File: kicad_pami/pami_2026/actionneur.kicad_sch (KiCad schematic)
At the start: 18 parts, among them J1 Conn_01x04_Socket, J10 Conn_01x07_Socket, J11 Conn_01x06, J12 Conn_01x06, J14 Conn_01x03_Pin, J2 Conn_01x03_Pin, J7 Conn_01x03_Pin, Q2 NMOS, Q3 NMOS, U1 DRV8833RTY

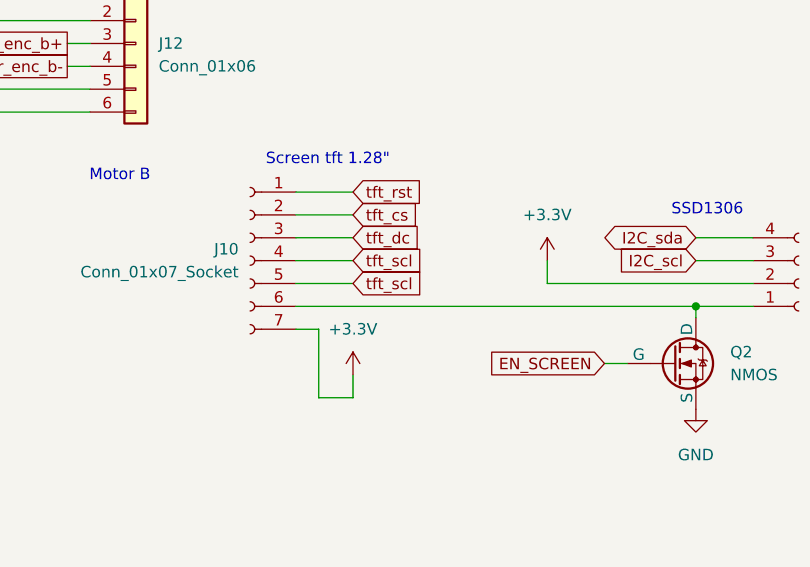
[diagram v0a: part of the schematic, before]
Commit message: ajout code / avancement pcb et 3D
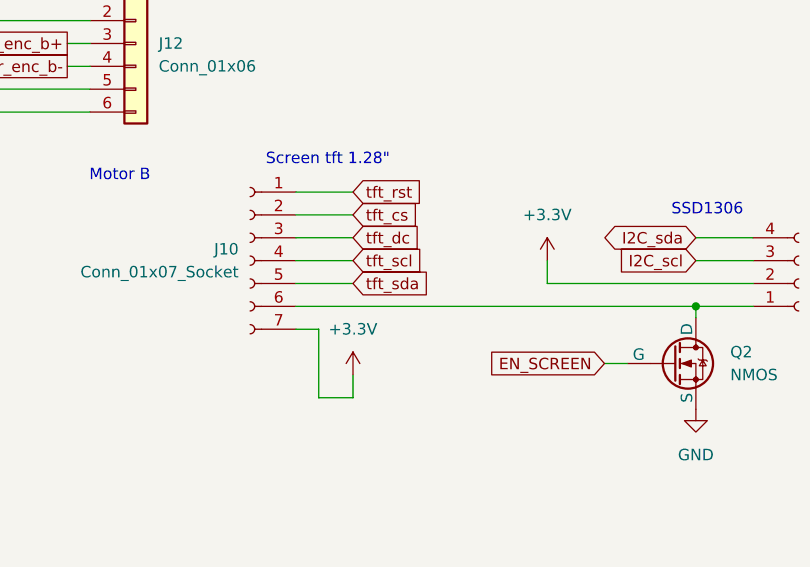
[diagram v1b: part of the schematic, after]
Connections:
- net tft_scl: no longer J10.5 (Pin_5)
- new net tft_sda: J10.5 (Pin_5)
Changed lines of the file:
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@@
 		)
 	)
-	(global_label "tft_scl"
+	(global_label "tft_sda"
 		(shape input)
 		(at 186.69 116.84 0)
@@
 		)
 		(property "Intersheetrefs" "${INTERSHEET_REFS}"
-			(at 195.6018 116.84 0)
+			(at 196.146 116.84 0)
 			(effects
 				(font

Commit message: fin PCB
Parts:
- D8: footprint LED_SMD:LED_SK6812MINI_PLCC4_3.5x3.5mm_P1.75mm -> CustomLibrary:IN-PI33TBTPRPGPB
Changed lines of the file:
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@@
 			)
 		)
-		(property "Footprint" "LED_SMD:LED_SK6812MINI_PLCC4_3.5x3.5mm_P1.75mm"
+		(property "Footprint" "CustomLibrary:IN-PI33TBTPRPGPB"
 			(at 121.92 185.42 0)
 			(effects
